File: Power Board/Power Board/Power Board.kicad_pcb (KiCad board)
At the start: 2 copper layers, 83.8 x 88.9 mm, 15 parts, among them J1 MINIFIT-2-VERT, J10 MINIFIT-2-VERT, J2 MINIFIT-2-VERT, J3 MINIFIT-2-VERT, J4 MEGAFIT-2-VERT, J5 MINIFIT-2-VERT, J6 MINIFIT-2-VERT, J7 MINIFIT-2-VERT, J8 MINIFIT-2-VERT, J9 MINIFIT-2-VERT

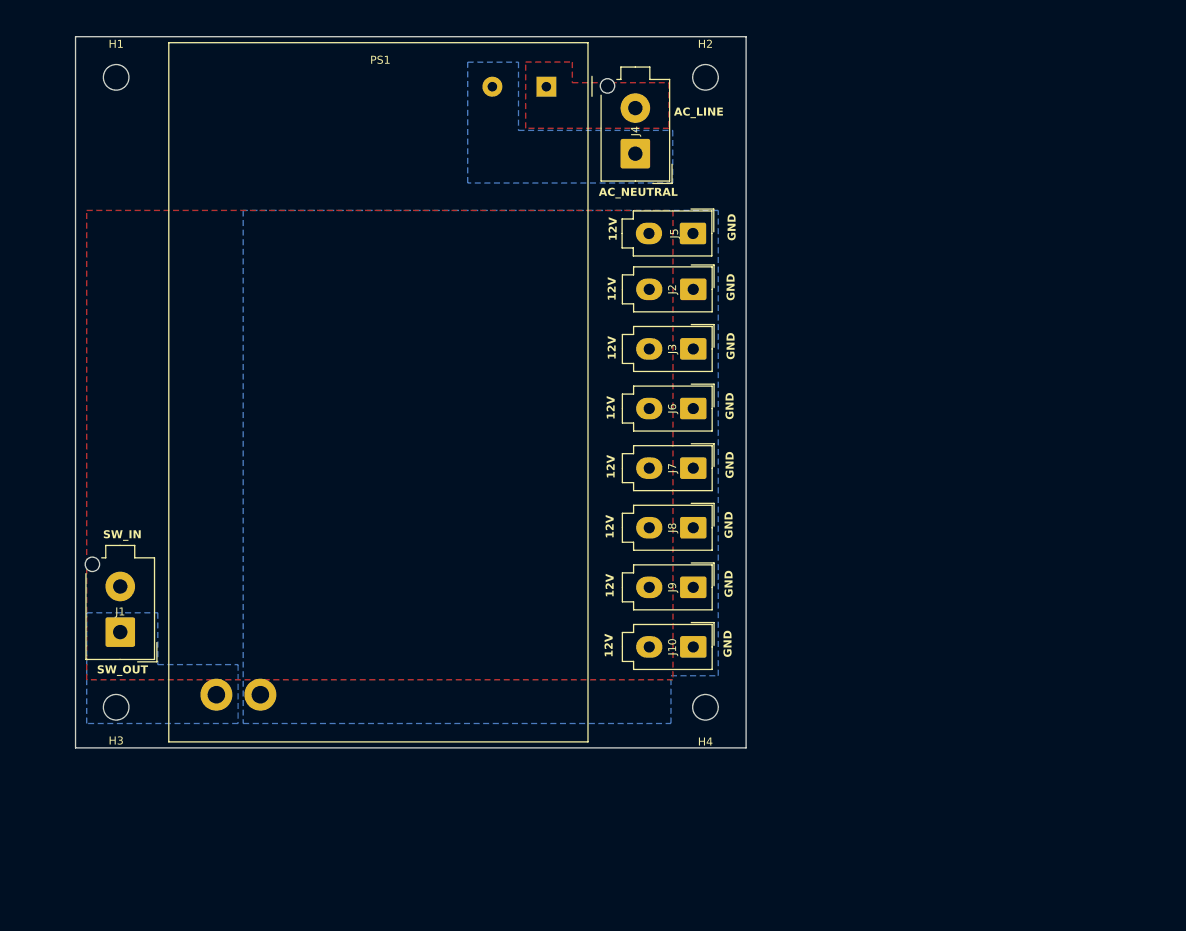
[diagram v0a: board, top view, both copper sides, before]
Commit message: Completed Power Board
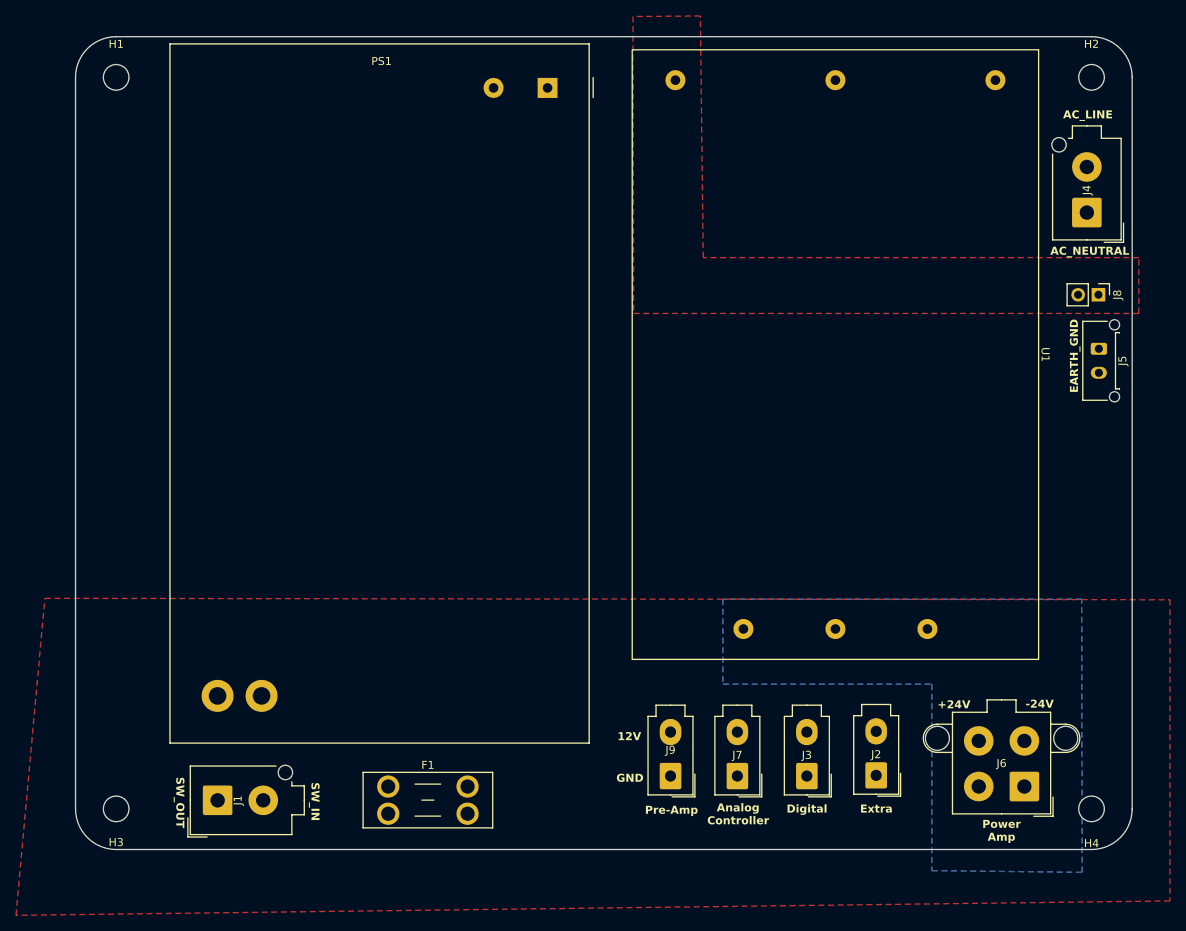
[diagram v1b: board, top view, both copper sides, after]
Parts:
- removed J10: MINIFIT-2-VERT, Connector_Molex:Molex_Mini-Fit_Jr_5566-02A_2x01_P4.20mm_Vertical
- added F1: Fuse, Fuse:Fuseholder_Blade_Mini_Keystone_3568, F.Cu at (64.5, 119.1)
- added U1: AC025-D24, GTSR_KiCAD_Footprints:AC025-D15, F.Cu at (145.8, 27.0)
- J5: footprint Connector_Molex:Molex_Mini-Fit_Jr_5566-02A_2x01_P4.20mm_Vertical -> Connector_Molex:Molex_Micro-Fit_3.0_43650-0215_1x02_P3.00mm_Vertical
- J6: value MINIFIT-2-VERT -> ~; footprint Connector_Molex:Molex_Mini-Fit_Jr_5566-02A_2x01_P4.20mm_Vertical -> Connector_Molex:Molex_Mega-Fit_76829-0004_2x02_P5.70mm_Vertical
- J8: footprint Connector_Molex:Molex_Mini-Fit_Jr_5566-02A_2x01_P4.20mm_Vertical -> Connector_PinHeader_2.54mm:PinHeader_1x02_P2.54mm_Vertical
- moved J2 64.9 mm to (125.5, 117.7), turned to 180 degrees
- moved J6 62.8 mm to (144.0, 119.1), turned to 180 degrees
- moved J8 58.4 mm to (153.3, 57.7)
- moved J4 56.9 mm to (151.8, 47.4)
- moved J3 55.2 mm to (116.8, 117.8), turned to 180 degrees
- moved J5 52.7 mm to (153.3, 64.4)
- moved H4 49.9 mm to (152.4, 121.9)
- moved H2 48.3 mm to (152.4, 30.5)
- moved J7 38.9 mm to (108.1, 117.8), turned to 180 degrees
- moved J1 24.3 mm to (43.2, 120.9), turned to 90 degrees
- moved J9 23.8 mm to (99.8, 117.8), turned to 180 degrees
- moved H3 12.7 mm to (30.5, 121.9)
- moved PS1 0.21 mm to (84.4, 31.8)
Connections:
- J1 pad 2: +12V -> Net-(F1-Pad1)
- J5 pad 1: GND -> /Earth_GND
- J5 pad 2: +12V -> /Earth_GND
- J6 pad 2: +12V -> GND
- J8 pad 1: GND -> /Earth_GND
- J8 pad 2: +12V -> Net-(U1-Frame_GND)
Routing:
- added copper zone on In1.Cu, net +12V
- added copper zone on In2.Cu, net +24V
- added copper zone on B.Cu, net -24V
- added copper zone on In2.Cu, net /AC_Line
- added copper zone on In1.Cu, net /AC_Neutral
- added copper zone on In1.Cu, net /Earth_GND
- added copper zone on F.Cu, net GND
- added copper zone on In2.Cu, net Net-(F1-Pad1)
- added copper zone on In1.Cu, net Net-(PS1-+Vout)
- added copper zone on F.Cu, net Net-(U1-Frame_GND)
- removed copper zone on F.Cu, net +12V
- removed copper zone on F.Cu, net /AC_Line
- removed copper zone on B.Cu, net /AC_Neutral
- removed copper zone on B.Cu, net GND
- removed copper zone on B.Cu, net Net-(PS1-+Vout)
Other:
- board size 83.8 x 88.9 mm -> 132.1 x 101.6 mm
- copper layers 2 -> 4
- board text added: "+24V"
- board text added: "-24V"
- board text added: "Analog Controller"
- board text added: "Digital"
- board text added: "EARTH_GND"
- board text added: "Extra"
- board text added: "Power Amp"
- board text added: "Pre-Amp"
